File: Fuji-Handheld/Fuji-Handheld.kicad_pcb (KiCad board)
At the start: 2 copper layers, 67.6 x 96.4 mm, 33 parts, among them J1 USB_C_Receptacle_USB2.0_16P, J2 Conn_01x02_Pin, J3 Conn_01x08_Pin, SW1 SW_SPDT, SW2 SW_Push, SW3 SW_Push, SW4 SW_Push, SW5 SW_Push, SW6 SW_Push, SW7 SW_Push, SW8 SW_Push, SW9 SW_Push, U1 MCP73831-2-OT, U2 AP2112K-3.3, U3 ESP32-S3-MINI-1

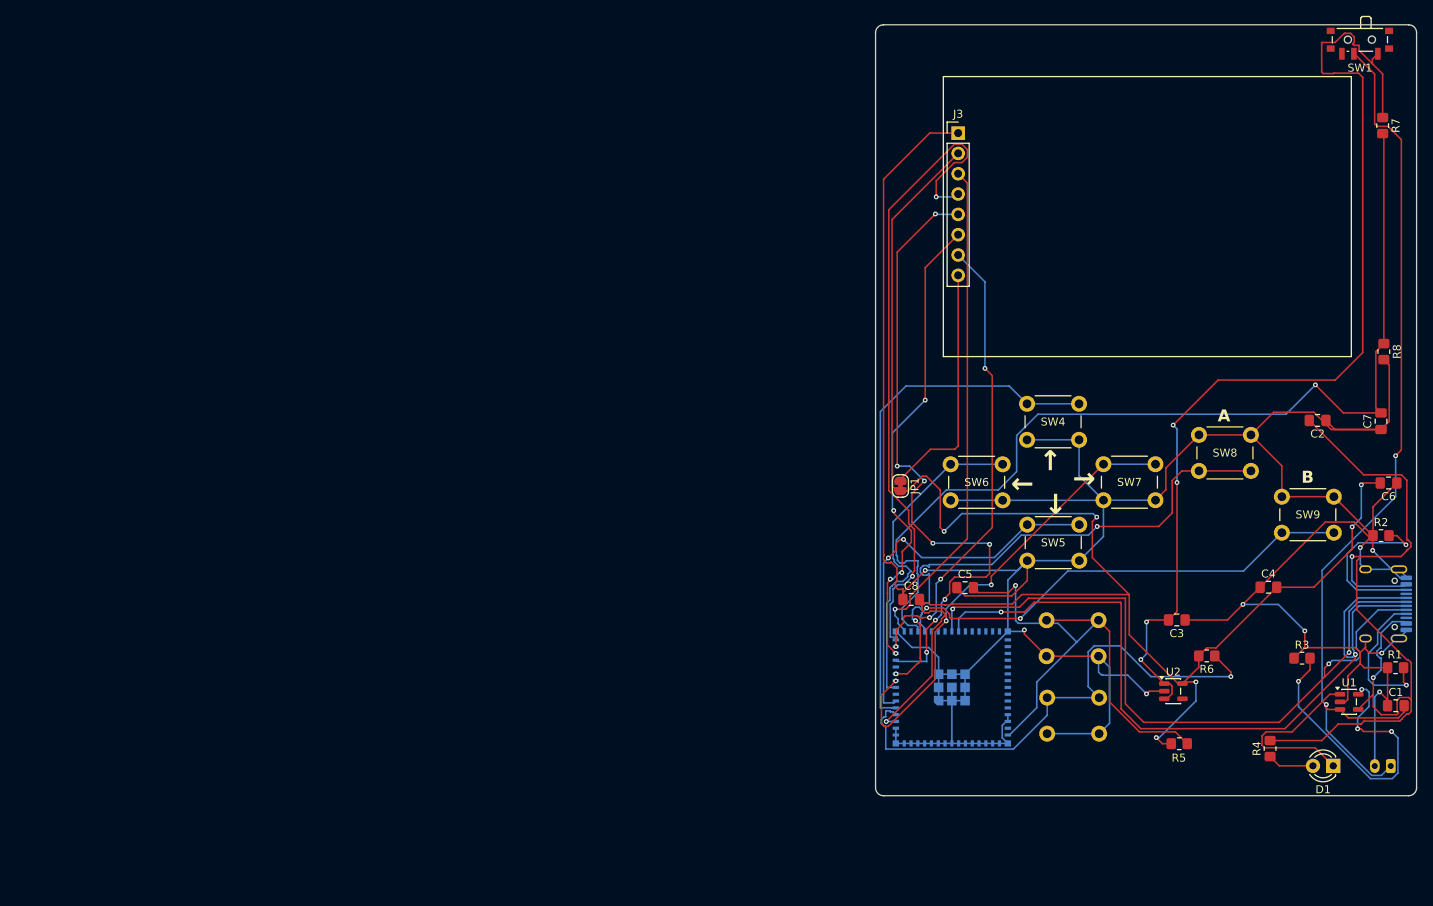
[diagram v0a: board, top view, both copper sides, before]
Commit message: Finished with the pcb / gerber files
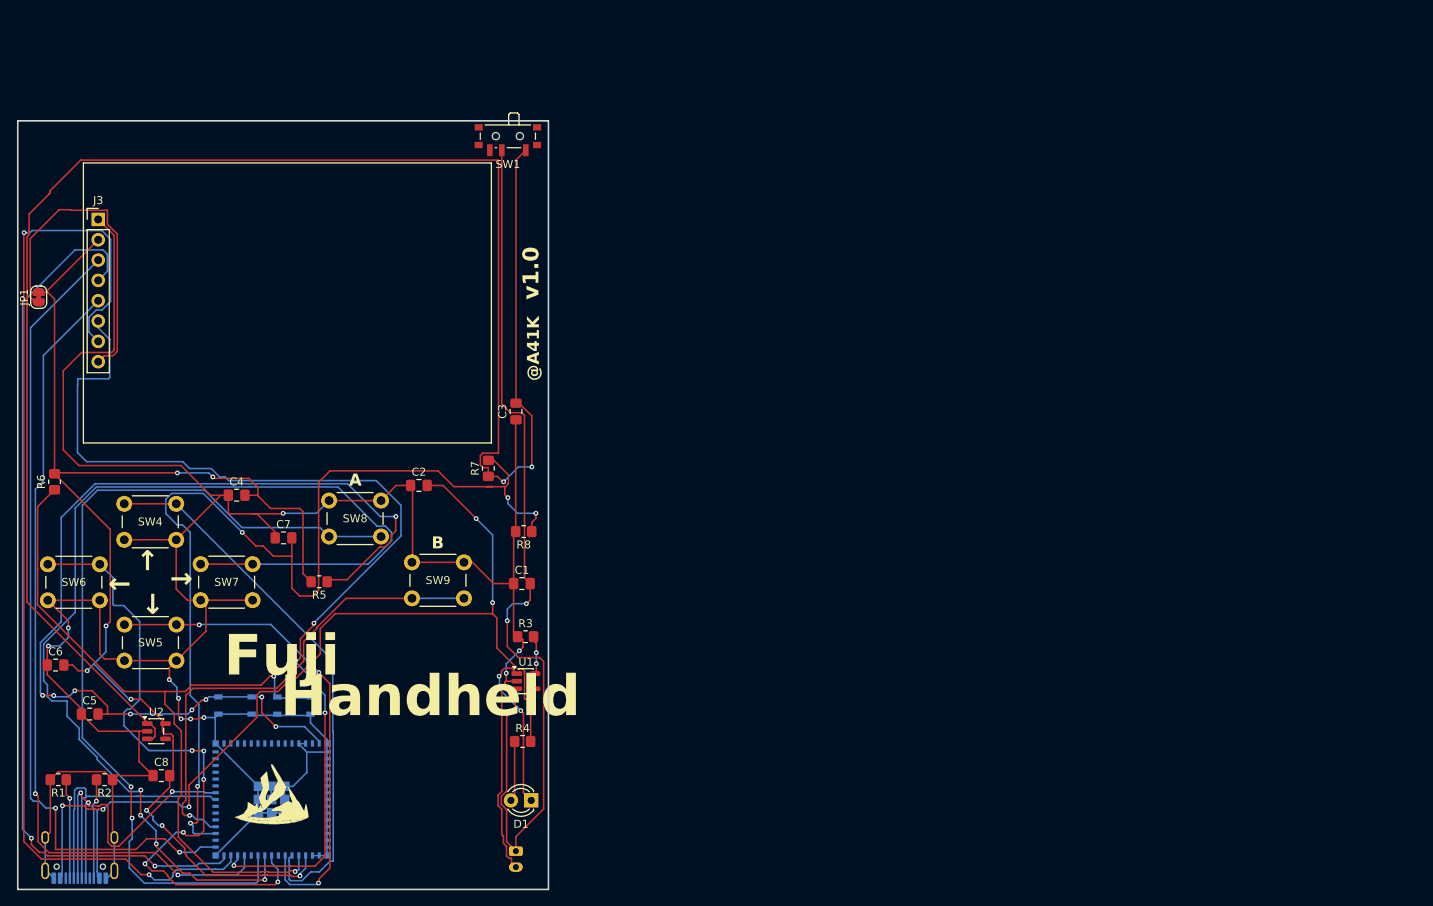
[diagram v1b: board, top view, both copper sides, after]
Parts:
- added G***: LOGO, LOGO, F.Cu at (92.0, 161.7)
- SW2, SW3: footprint Button_Switch_THT:SW_PUSH_6mm_H4.3mm -> Button_Switch_SMD:SW_SPST_PTS810
- moved C6 168.2 mm to (65.0, 146.4), turned to 0 degrees
- moved R1 167.7 mm to (65.4, 160.8)
- moved J1 164.6 mm to (68.1, 169.0), turned to 0 degrees
- moved R2 162.4 mm to (71.2, 160.8), turned to 180 degrees
- moved R6 145.7 mm to (64.9, 123.5), turned to 90 degrees
- moved C7 138.0 mm to (93.5, 130.5), turned to 0 degrees
- moved C4 129.5 mm to (87.7, 125.2)
- moved U2 127.2 mm to (77.6, 154.7)
- moved R7 119.7 mm to (119.1, 121.8), turned to 90 degrees
- moved SW4 113.5 mm to (73.6, 126.3)
- moved SW5 113.5 mm to (73.6, 141.4)
- moved SW7 113.5 mm to (83.2, 133.8)
- moved SW6 113.5 mm to (64.1, 133.8)
- moved C2 112.6 mm to (110.4, 124.0), turned to 0 degrees
- moved C5 110.6 mm to (69.3, 152.6)
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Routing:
- net VSYS: track 129.7 -> 225.1 mm, vias 4 -> 2
- net BTN_RIGHT: track 59.1 -> 139.9 mm, vias 3 -> 4
- net TFT_CS: track 58.0 -> 132.1 mm, vias 4 -> 2
- net TFT_DC: track 58.9 -> 128.5 mm, vias 5 -> 4
- net USB_DN: track 100.4 -> 41.4 mm, vias 3 -> 0
- net Net-(U3-EN): track 67.4 -> 124.7 mm, vias 1 -> 9
- net USB_DP: track 98.4 -> 46.5 mm, vias 2 -> 3
- net GND: track 448.3 -> 400.3 mm, vias 9 -> 10
- net +3V3: track 207.3 -> 162.6 mm, vias 7 -> 8
- net BTN_LEFT: track 41.9 -> 82.8 mm, vias 0 -> 6
- net BTN_A: track 68.3 -> 108.8 mm, vias 3 -> 2
- net TFT_SCLK: track 62.7 -> 101.1 mm, vias 1 -> 2
- net Net-(U1-PROG): track 40.0 -> 4.82 mm, vias 4 -> 2
- net TFT_MOSI: track 82.5 -> 111.6 mm
- net Net-(U3-IO0): track 67.0 -> 95.7 mm, vias 1 -> 2
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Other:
- board size 67.6 x 96.4 mm -> 66.3 x 96.1 mm
- board text added: "@A41K"
- board text added: "Fuji"
- board text added: "Handheld"
- board text added: "v1.0"
